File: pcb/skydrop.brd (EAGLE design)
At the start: 103 x 83 mm, 98 parts, among them IC1 RT9193-33GB, IC2 MCP73831/OT, IC3 STM809SWX6F, IC4 MS5611-01BA03, Q1 BSS84, Q10 BSS84, Q2 BSS123, Q3 BSS123, Q4 BSS84, Q5 BSS84, Q6 BSS84, Q7 BSS123, Q8 BSS84, Q9 BSS84, U2 W25Q16BVSS

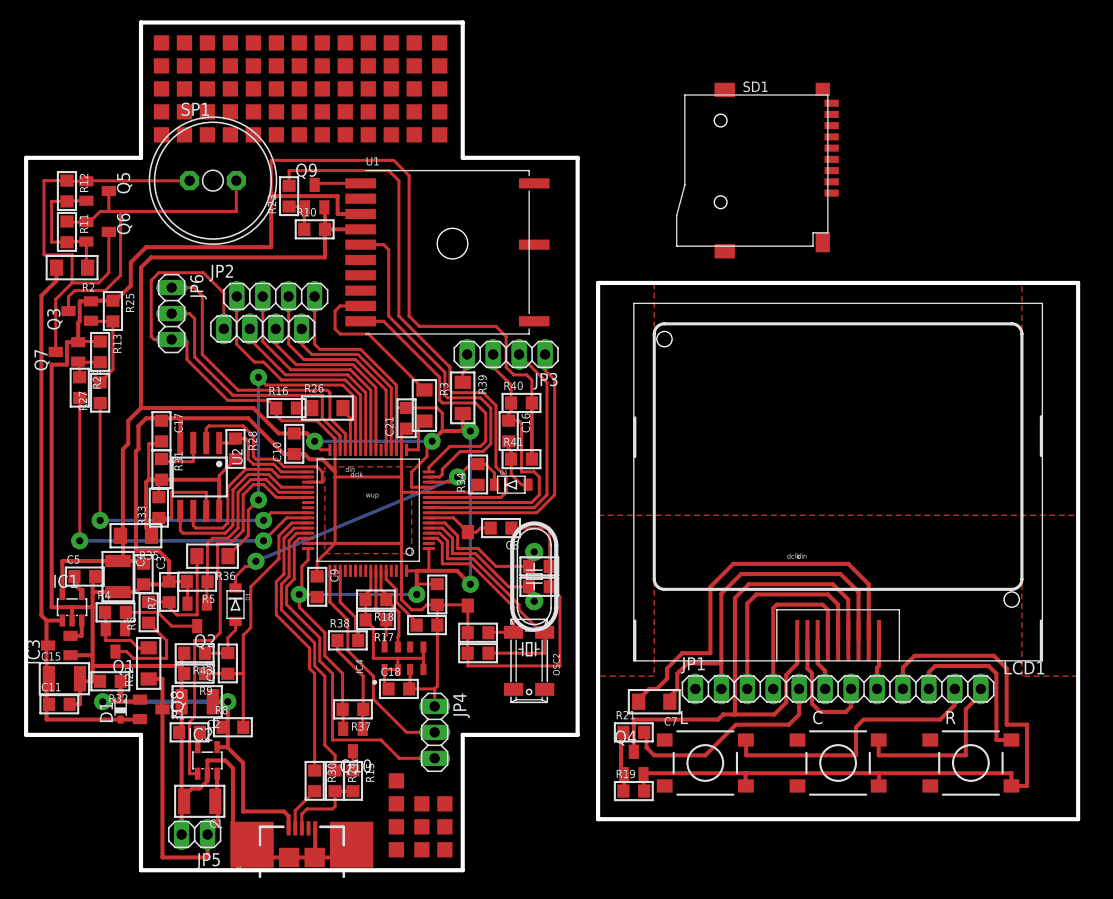
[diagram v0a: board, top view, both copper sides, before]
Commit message: [pcb] new display
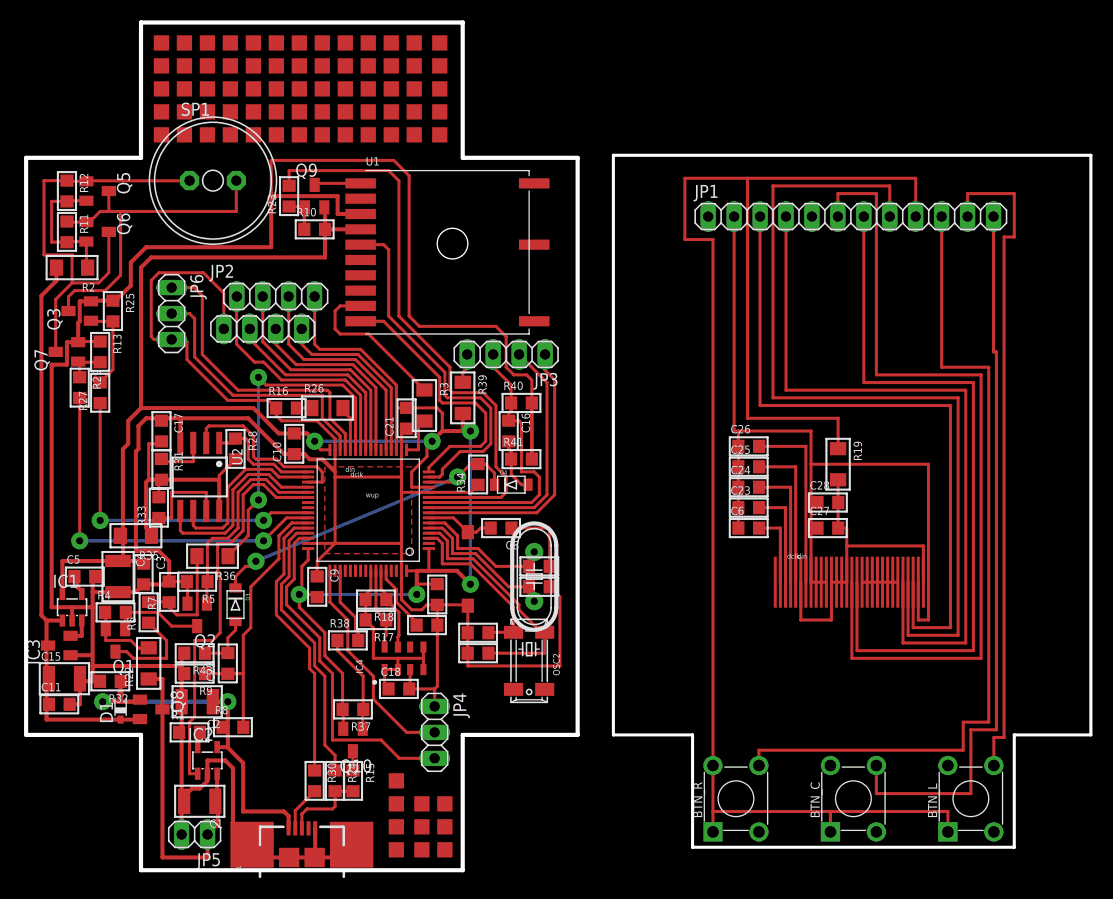
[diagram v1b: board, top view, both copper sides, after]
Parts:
- removed C, L, R: DTSM-6, skydrop:DTSM-6
- removed C7: (no value), skydrop:C1206
- removed LCD1: LPH-7366, skydrop:LPH-7366
- removed Q4: BSS84, transistor-small-signal:SOT23
- removed R21: 100, skydrop:R0805
- removed SD1: TF-HOLDER, skydrop:TF-PULL
- added BTN_C, BTN_L, BTN_R: TS-1109-7, skydrop:SW4-6.2X6.2X5.0MM
- added C23, C24, C25, C6: 1uf, skydrop:C0805
- added C26: 3.3uf, skydrop:C0805
- added C27: 0.1uf, skydrop:C0805
- added C28: 10uf, skydrop:C0805
- added U$1: NOKIA5110, skydrop:NOKIA5110
- R19: value 10k -> 0; device skydrop:R0805 -> skydrop:R1206
- moved JP1 46.3 mm to (83.2, 64.5)
- moved R19 37.7 mm to (82.0, 40.2), turned to 270 degrees
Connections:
- removed net N$26: Q4.1, R19.1, R21.1
- removed net VDD: SD1.4
- removed net VSS: SD1.6
- new net N$15: C27.2, C28.2, R19.2, U$1.10, U$1.11, U$1.12, U$1.13, U$1.14, U$1.17, U$1.18, U$1.19, U$1.2, U$1.20, U$1.26, U$1.7, U$1.8, U$1.9
- new net N$40: C6.2, U$1.30
- new net N$47: C23.2, U$1.29
- new net N$48: C24.2, U$1.28
- new net N$49: C25.2, U$1.27
- new net N$50: C26.2, U$1.25
- new net N$52: BTN_R.2
- net BTN_C_T: now also BTN_C.3; no longer C.2
- net BTN_L_T: now also BTN_L.3; no longer L.2
- net BTN_R_T: now also BTN_R.3; no longer R.2
- net GND_T: now also C23.1, C24.1, C25.1, C26.1, C27.1, C28.1, C6.1, U$1.1, U$1.21, U$1.22, U$1.23, U$1.24, U$1.3; no longer C7.1, LCD1.7
- net LCD_CE_T: now also U$1.4; no longer LCD1.5
- net LCD_CLK_T: now also U$1.15; no longer LCD1.2
- net LCD_DC_T: now also U$1.6; no longer LCD1.4
- net LCD_DIN_T: now also U$1.16; no longer LCD1.3
- net LCD_PWR_T: no longer R21.2
- net LCD_RST_T: now also U$1.5; no longer LCD1.9
- net N$25: now also BTN_L.2; no longer LCD1.1, LCD1.6, Q4.3
- net N$36: now also BTN_C.2; no longer C7.2, LCD1.8
- net VCC_T: now also BTN_C.1, BTN_C.4, BTN_L.1, BTN_L.4, BTN_R.1, BTN_R.4, R19.1; no longer C.4, L.4, Q4.2, R.4, R19.2
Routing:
- net VCC_T: track 69.8 -> 155.5 mm
- net LCD_RST_T: track 4.83 -> 86.7 mm
- net LCD_DIN_T: track 5.05 -> 81.9 mm
- net BTN_R_T: track 16.8 -> 80.9 mm
- net LCD_CLK_T: track 12.5 -> 71.3 mm
- net LCD_DC_T: track 16.6 -> 71.5 mm
- net BTN_C_T: track 17.1 -> 71.3 mm
- net N$25: track 53.0 -> 0.00 mm
- net GND_T: track 36.8 -> 85.8 mm
- net LCD_CE_T: track 21.5 -> 67.0 mm
- net N$36: track 39.0 -> 0.00 mm
- net BTN_L_T: track 27.2 -> 64.8 mm
- net N$15: track 0.00 -> 37.3 mm
- net LCD_PWR_T: track 21.0 -> 0.00 mm
- net N$50: track 0.00 -> 17.9 mm
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- removed copper zone on layer 1, net N$15
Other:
- board size 103 x 83 mm -> 104.2 x 83 mm
